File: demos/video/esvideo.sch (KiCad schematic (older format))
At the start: 29 parts, among them U8 BT253, U9 BT473

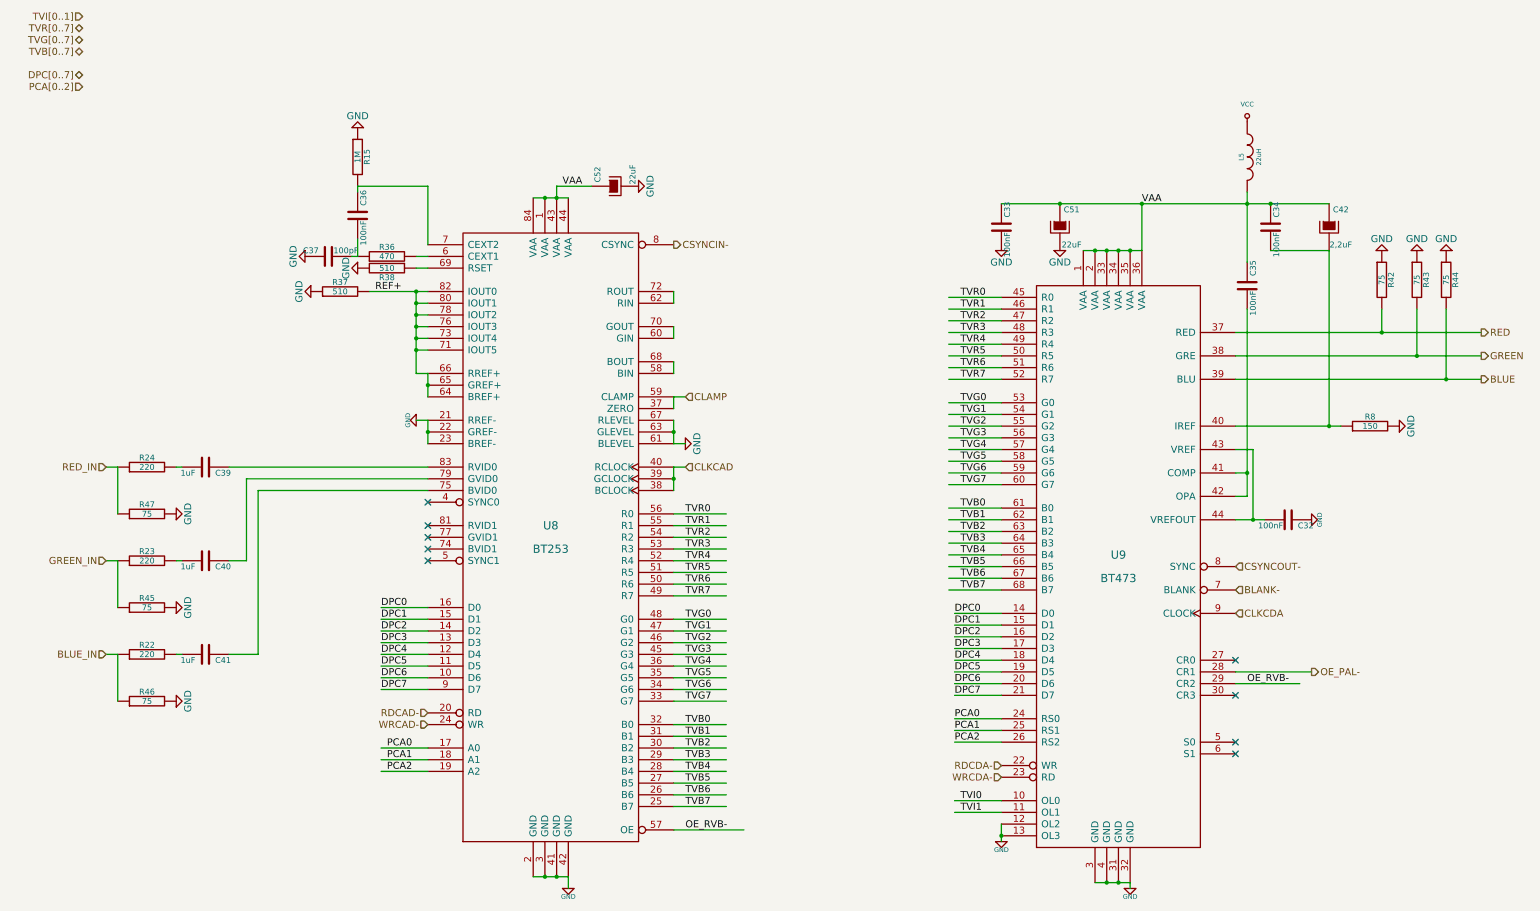
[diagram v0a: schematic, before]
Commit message: Imported Upstream version 4.0.0~rc1
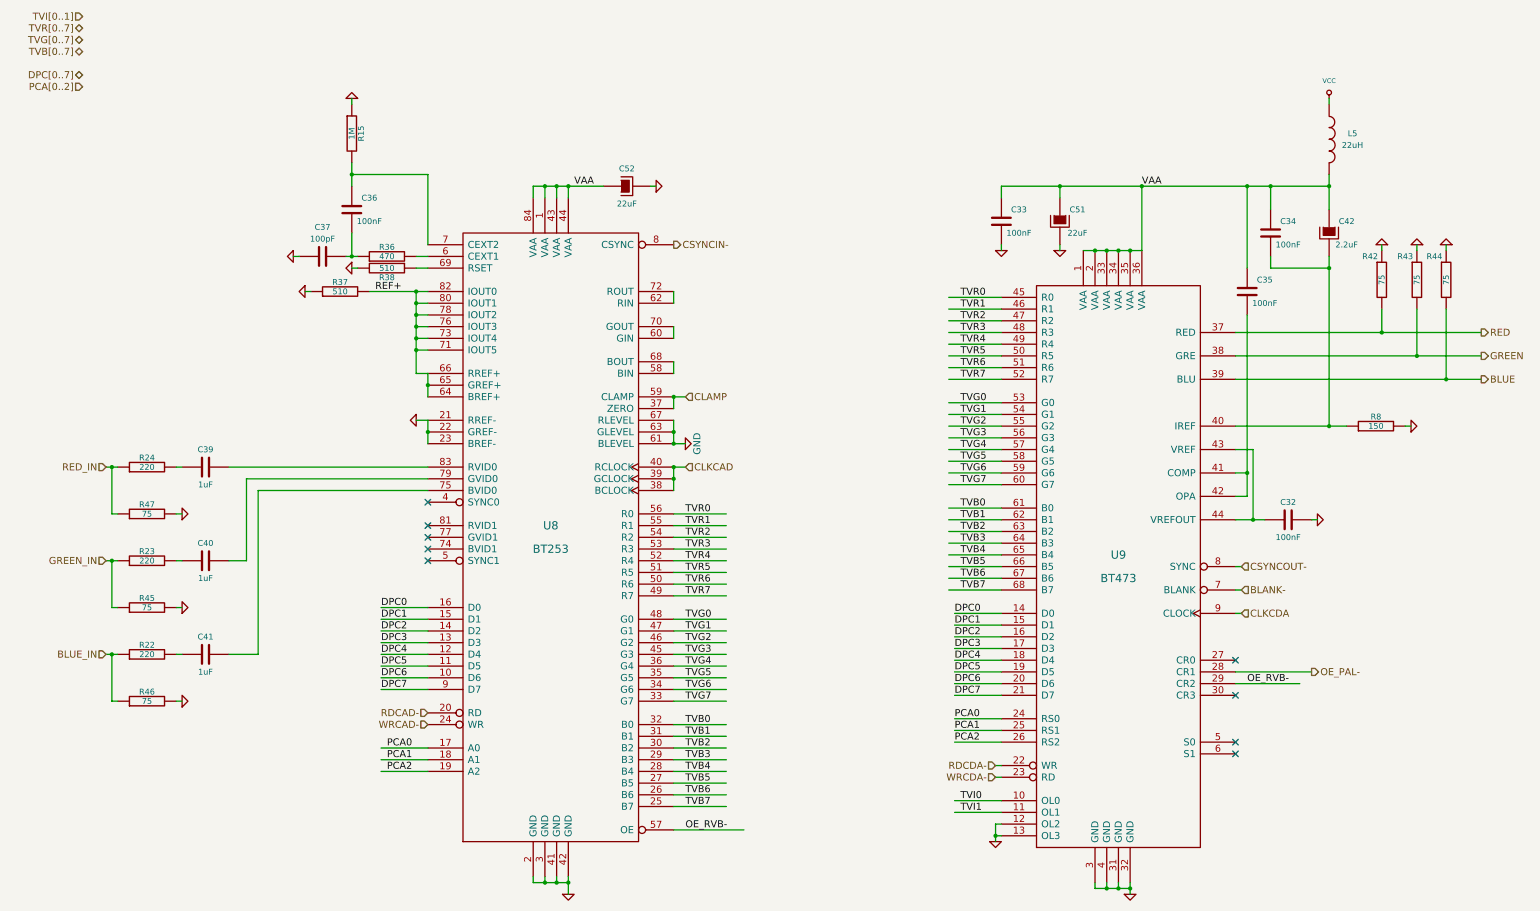
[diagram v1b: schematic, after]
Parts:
- C32, C33, C34, C35, C36, C37, C52, R15, R22, R23, R24, R36, R37, R38, R42, R43, R44, R45, R46, R47, R8: footprint (none) -> lib_smd:SM1206
- C39, C40, C41, C51: footprint (none) -> lib_smd:SM1210L
- C42: value 2,2uF -> 2.2uF; footprint (none) -> lib_smd:SM1210L
- L5: footprint (none) -> lib_smd:SM1812
- U8: footprint (none) -> footprints:PLCC84
- U9: footprint (none) -> footprints:PLCC68
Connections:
- wire segments 145 -> 184
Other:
- moved on the sheet: C33, C34, C35, C36, C37, C42, C51, C52, L5, R15, R8
